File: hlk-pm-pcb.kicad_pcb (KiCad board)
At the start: 2 copper layers, 12 parts, among them J1 AC-In, J2 DC-Out

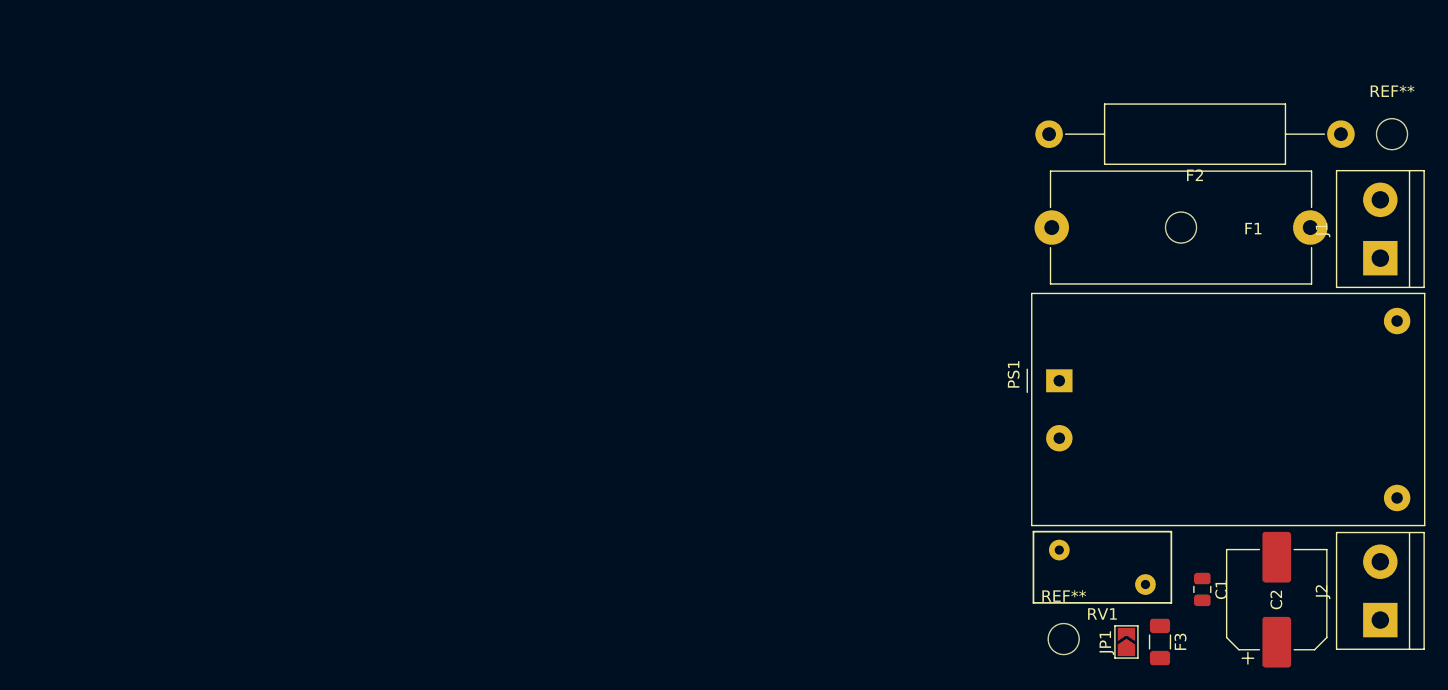
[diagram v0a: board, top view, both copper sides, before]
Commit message: development
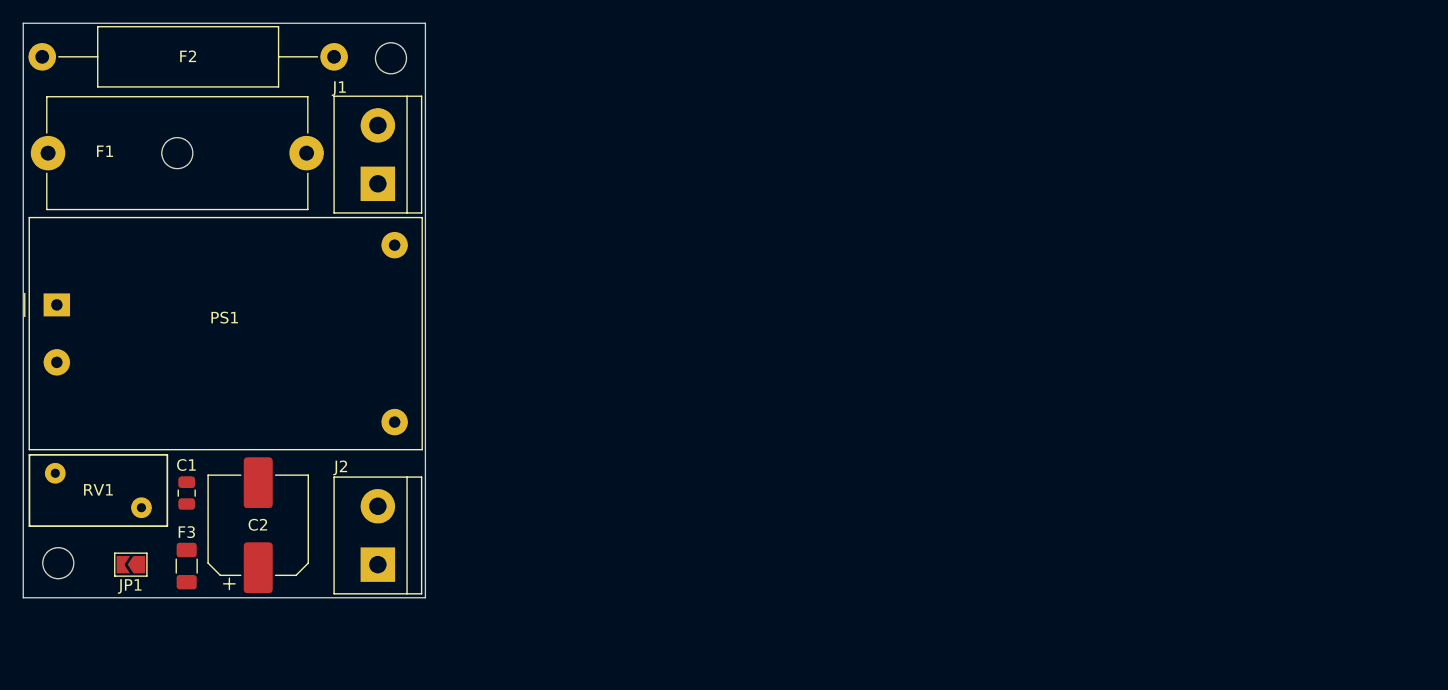
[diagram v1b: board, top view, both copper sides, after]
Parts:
- moved F1 110.0 mm to (78.5, 62.0), turned to 0 degrees
- moved C2 88.9 mm to (96.8, 94.4)
- moved C1 88.8 mm to (90.6, 91.6), turned to 90 degrees
- moved F2 87.9 mm to (103.4, 53.6)
- moved REF** 87.8 mm to (79.4, 97.7)
- moved PS1 87.5 mm to (79.2, 75.2)
- moved J1 87.5 mm to (107.2, 64.6)
- moved J2 87.4 mm to (107.2, 97.8)
- moved REF** 87.4 mm to (108.3, 53.7)
- moved JP1 86.9 mm to (85.7, 97.8), turned to 180 degrees
- moved F3 85.0 mm to (90.6, 97.9)
- moved RV1 80.0 mm to (86.6, 92.8), turned to 180 degrees
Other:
- board outline added: 35 x 50 mm

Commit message: Release board v.1.0
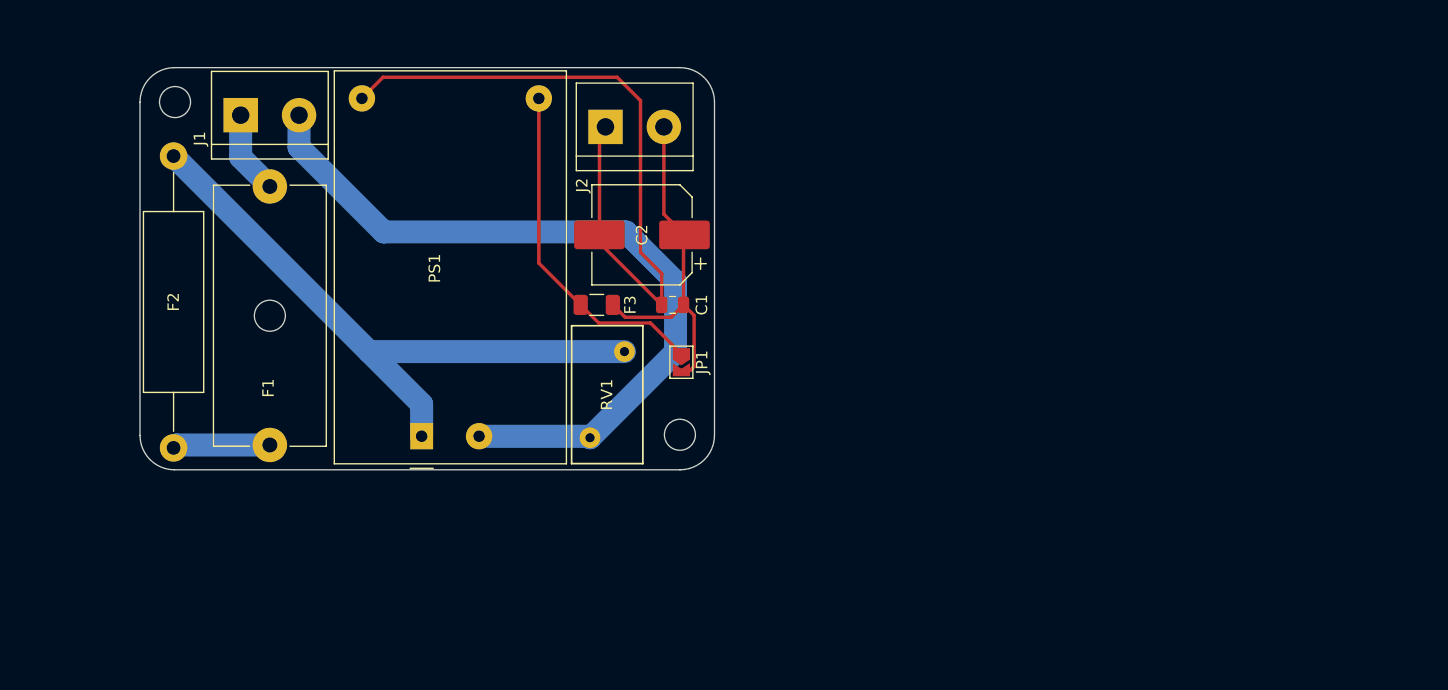
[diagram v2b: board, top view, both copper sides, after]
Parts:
- added G***: LOGO, logo:d-diot-logo, B.Cu at (112.5, 69.6)
- F3: value Fuse -> Fuse 1.5A
- moved REF** 55.2 mm to (133.5, 86.5), turned to 90 degrees
- moved JP1 51.1 mm to (133.6, 80.2), turned to 270 degrees
- moved C1 45.4 mm to (132.8, 75.2), turned to 180 degrees
- moved RV1 44.2 mm to (128.7, 79.2), turned to 270 degrees
- moved J2 42.9 mm to (127.0, 59.7), turned to 0 degrees
- moved F3 42.3 mm to (126.2, 75.2), turned to 180 degrees
- moved C2 41.9 mm to (130.2, 69.1), turned to 180 degrees
- moved PS1 33.7 mm to (111.0, 86.6), turned to 90 degrees
- moved F1 31.9 mm to (97.8, 87.4), turned to 90 degrees
- moved REF** 19.2 mm to (89.5, 57.5), turned to 90 degrees
- moved F2 16.4 mm to (89.4, 62.2), turned to 270 degrees
- moved J1 13.3 mm to (95.2, 58.7), turned to 0 degrees
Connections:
- J1 pad 1: Net-(J1-Pad1) -> Net-(F1-Pad2)
- J1 pad 2: Net-(F1-Pad2) -> Net-(J1-Pad2)
- J2 pad 1: Net-(C1-Pad1) -> Net-(C1-Pad2)
- J2 pad 2: Net-(C1-Pad2) -> Net-(C1-Pad1)
- PS1 pad 2: Net-(J1-Pad1) -> Net-(J1-Pad2)
- RV1 pad 2: Net-(J1-Pad1) -> Net-(J1-Pad2)
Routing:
- net Net-(J1-Pad2): track 0.00 -> 66.8 mm
- net Net-(C1-Pad2): track 0.00 -> 62.4 mm
- net Net-(F2-Pad1): track 0.00 -> 55.6 mm
- net Net-(C1-Pad1): track 0.00 -> 32.7 mm
- net Net-(F3-Pad2): track 0.00 -> 30.5 mm
- net Net-(F1-Pad1): track 0.00 -> 8.49 mm
- net Net-(F1-Pad2): track 0.00 -> 7.25 mm
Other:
- board size 35 x 50 mm -> 50 x 35 mm
- net class Default: trace_width 0.25 -> 0.16; via_dia 0.8 -> 0.65; via_drill 0.4 -> 0.35
- rule trace_min: 0.2 -> 0.16
- rule via_min_drill: 0.3 -> 0.35
- rule via_min_size: 0.4 -> 0.65
- board text added: "HLK-PM Pcb - v.1.0"
